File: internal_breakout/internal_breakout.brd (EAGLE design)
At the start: 50 x 35 mm, 21 parts, among them J10 2X5, J11 2X5, J3 2X5, J4 2X5, Q1 DMP3099L, U1 LP2985

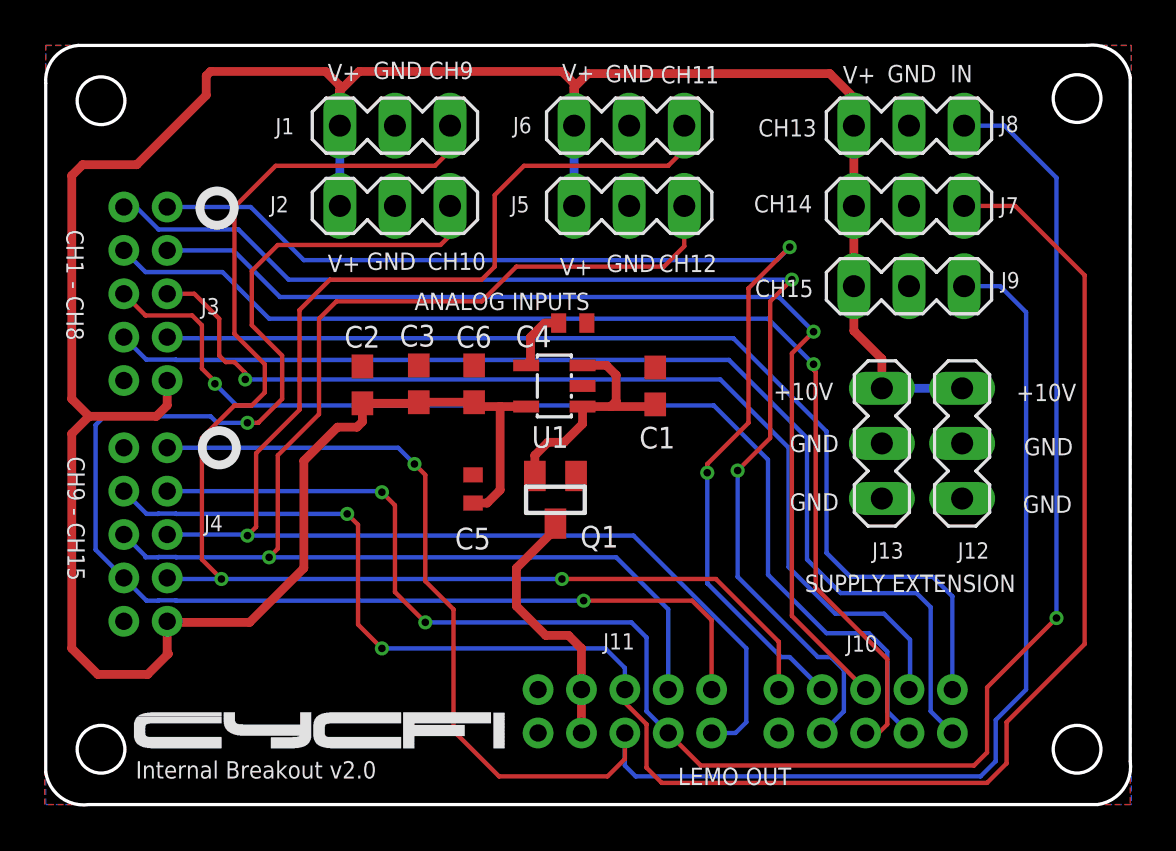
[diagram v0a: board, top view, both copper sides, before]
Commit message: push updated files for internal breakout
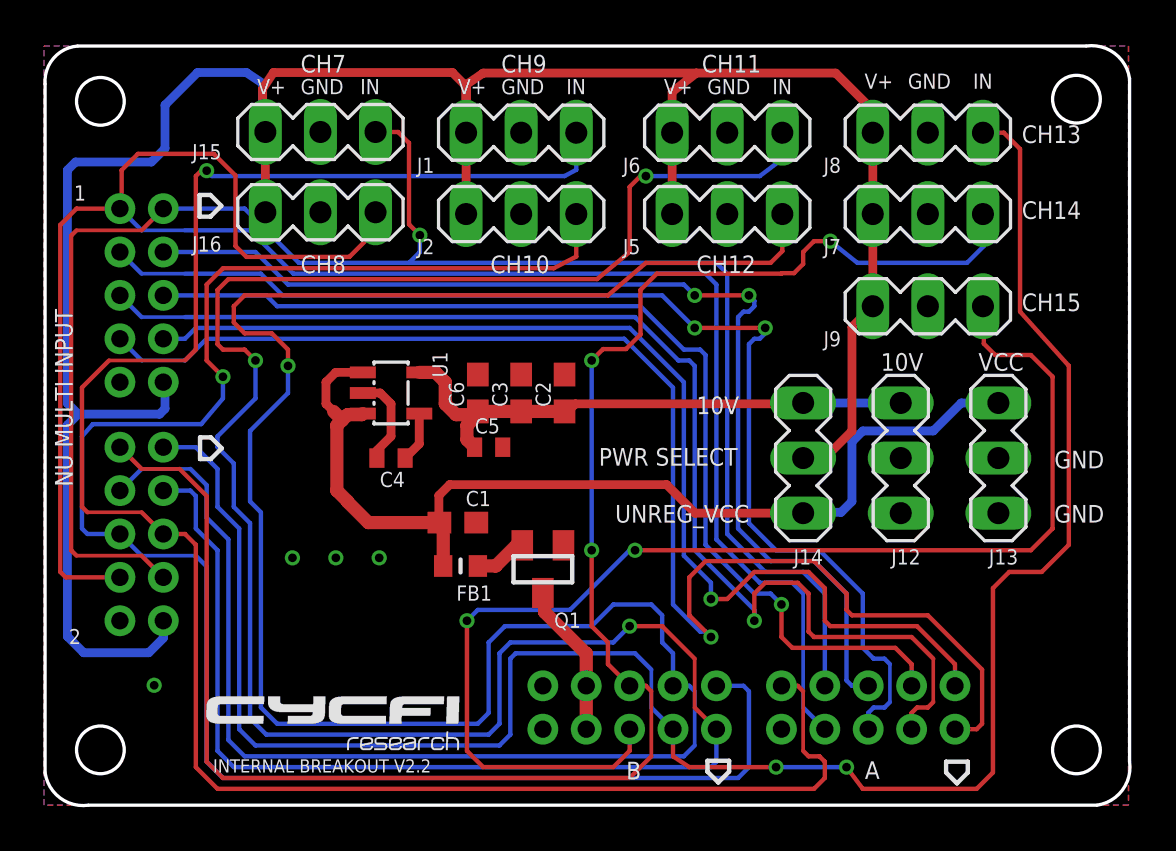
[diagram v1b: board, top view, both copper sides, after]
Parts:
- added FB1: BLM18KG700TN1D, SamacSys_Parts:BEADC1608X75N
- added J14, J15, J16: (no value), con-lstb:MA03-1
- C1: value 1uF -> 10uF
- moved C1 11.1 mm to (19.0, 13.0), turned to 0 degrees
- moved C4 10.4 mm to (15.9, 16.0), turned to 180 degrees
- moved C2 9.33 mm to (23.9, 19.0)
- moved U1 7.54 mm to (15.9, 19.0), turned to 270 degrees
- moved J2 5.83 mm to (21.9, 27.2)
- moved J1 5.83 mm to (21.9, 31.0)
- moved J13 5.41 mm to (43.9, 16.0)
- moved C3 4.74 mm to (21.9, 19.0)
- moved J5 4.54 mm to (31.4, 27.2)
- moved J6 4.53 mm to (31.4, 31.0)
- moved Q1 3.25 mm to (22.9, 10.9)
- moved J12 2.91 mm to (39.4, 16.0)
- moved C5 2.06 mm to (20.4, 16.5), turned to 0 degrees
- moved J9 1.27 mm to (40.7, 23.0)
- moved J7 0.95 mm to (40.7, 27.2)
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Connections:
- removed net NC: J4.2
- new net +10VA: C2.1, C3.1, C5.1, C6.1, J12.3, J14.3, U1.5
- new net VIN: J11.7, J11.8, Q1.3
- net CH10: now also J4.6; no longer J4.8
- net CH11: now also J4.3; no longer J4.5
- net CH12: now also J4.4; no longer J4.6
- net CH13: now also J4.1; no longer J4.3
- net CH14: now also J4.2; no longer J4.4
- net CH15: no longer J4.1
- net CH7: now also J15.3, J4.7
- net CH8: now also J16.3, J4.8
- net CH9: now also J4.5; no longer J4.7
- net GND: now also J15.2, J16.2
- net N$1: now also FB1.1; no longer C1.1, U1.1, U1.3
- net V+: now also J14.2, J15.1, J16.1; no longer C2.1, C3.1, C5.1, C6.1, J12.3, J13.3, U1.5
- net VCC: now also C1.1, FB1.2, J13.3, J14.1, U1.1, U1.3; no longer J11.7, J11.8, Q1.3
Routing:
- net CH12: track 62.3 -> 118.4 mm
- net CH11: track 69.3 -> 121.5 mm, vias 1 -> 3
- net CH8: track 56.9 -> 93.4 mm, vias 2 -> 0
- net VCC: track 12.3 -> 47.3 mm
- net CH9: track 63.6 -> 90.7 mm, vias 2 -> 1
- net CH7: track 54.4 -> 80.9 mm, vias 2 -> 1
- net +10VA: track 0.00 -> 25.8 mm
- net CH15: track 78.8 -> 56.4 mm, vias 1 -> 2
- net V+: track 136.2 -> 116.1 mm
- net CH10: track 65.7 -> 82.7 mm, vias 2 -> 1
- net CH13: track 80.7 -> 92.8 mm, vias 3 -> 2
- net CH2: track 51.9 -> 63.0 mm, vias 0 -> 1
- net N$1: track 11.2 -> 2.44 mm
- net VIN: track 0.00 -> 7.12 mm
- net CH4: track 50.5 -> 56.9 mm
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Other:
- board text added: "1"
- board text added: "10V"
- board text added: "2"
- board text added: "A"
- board text added: "B"
- board text added: "CH7"
- board text added: "CH8"
- board text added: "INTERNAL BREAKOUT V2.2"
- board text added: "J15"
- board text added: "J16"
- board text added: "NU MULTI INPUT"
- board text added: "PWR SELECT"
- board text added: "UNREG_VCC"
- board text added: "VCC"
- board text removed: "+10V"
- board text removed: "ANALOG INPUTS"
- board text removed: "CH1 - CH8"
- board text removed: "CH9 - CH15"
- board text removed: "Internal Breakout v2.0"
- board text removed: "J10"
- board text removed: "J11"
- board text removed: "J3"
- board text removed: "J4"
- board text removed: "LEMO OUT"
- board text removed: "SUPPLY EXTENSION"
